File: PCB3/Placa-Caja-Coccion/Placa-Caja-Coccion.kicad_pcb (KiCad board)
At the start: 2 copper layers, 49 x 67.8 mm, 41 parts, among them K1 G5LE-1, P1 RELAY_OUT, P2 MOSFET_OUT, P3 MOTOR1, P4 MOTOR_POWER, P5 HEADER1, P6 HEADER2, P7 MOTOR2, Q1 AOD4184A, Q2 S8050, U1 TB9051FTG, U2 TB9051FTG, U3 PC817

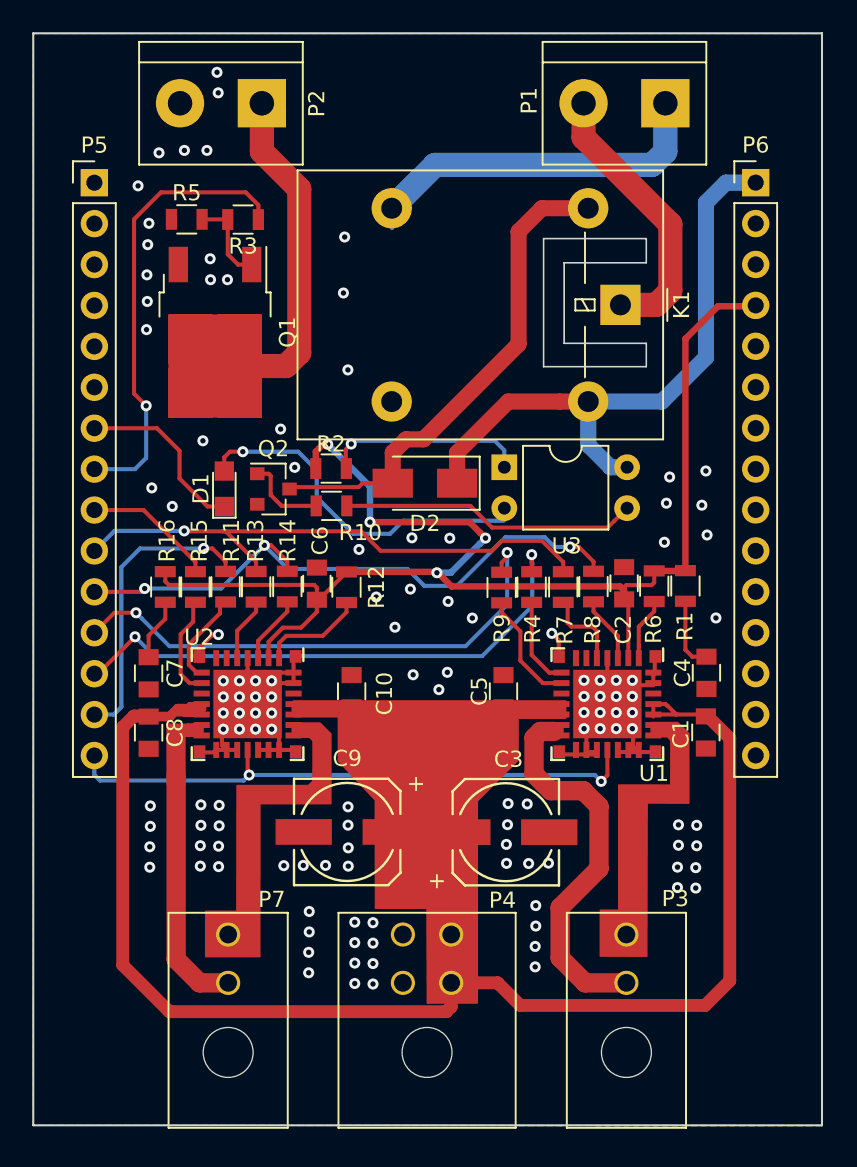
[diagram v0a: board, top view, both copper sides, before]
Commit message: Documentos de referencia actualizados
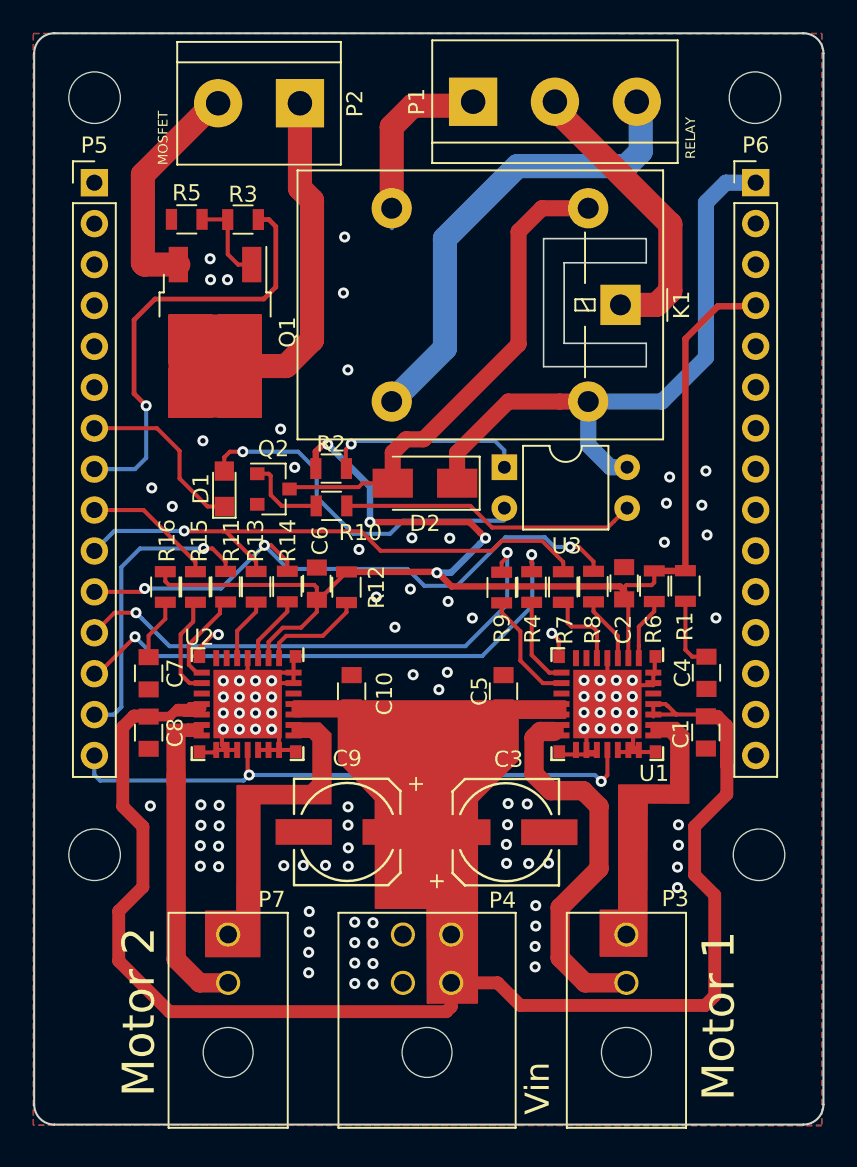
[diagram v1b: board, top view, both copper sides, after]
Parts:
- added G***: LOGO, logos_frizzy:logoWTF_small, B.Cu at (147.2, 119.8)
- added REF**: MountingHole_3.2mm_M3, Mounting_Holes:MountingHole_3.2mm_M3, F.Cu at (126.5, 119.5)
- added REF**: MountingHole_3.2mm_M3, Mounting_Holes:MountingHole_3.2mm_M3, F.Cu at (126.5, 72.5)
- added REF**: MountingHole_3.2mm_M3, Mounting_Holes:MountingHole_3.2mm_M3, F.Cu at (167.5, 72.5)
- added REF**: MountingHole_3.2mm_M3, Mounting_Holes:MountingHole_3.2mm_M3, F.Cu at (167.8, 119.5)
- P1: footprint TerminalBlock:TerminalBlock_bornier-2_P5.08mm -> TerminalBlock:TerminalBlock_bornier-3_P5.08mm
- moved P1 11.9 mm to (150.0, 72.8), turned to 0 degrees
- moved P2 2.36 mm to (139.2, 72.8)
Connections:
- P2 pad 2: GND -> GNDA
- Q1 pad 3: GND -> GNDA
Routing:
- net NC: track 0.00 -> 29.1 mm
- net NO: track 27.2 -> 12.9 mm
- net GNDA: track 0.00 -> 14.2 mm
- net VIN: track 132.2 -> 134.7 mm
- net MOSFET_SIG: track 28.3 -> 27.0 mm
- net COM: track 17.3 -> 18.2 mm
- net GND: vias 124 -> 106
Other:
- outline, holes or cut-outs redrawn
- board text added: "C"
- board text added: "GNDA"
- board text added: "MOSFET"
- board text added: "Motor 1"
- board text added: "Motor 2"
- board text added: "NC"
- board text added: "NO"
- board text added: "OUT-"
- board text added: "Placa Cocción V0.1"
- board text added: "RELAY"
- board text added: "Vin"
